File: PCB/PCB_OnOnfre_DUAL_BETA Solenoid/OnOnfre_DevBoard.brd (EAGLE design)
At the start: 44.1 x 43.8 mm, 29 parts, among them J1 9PIN 2.54MM, J3Y S8050, J7 8p, K1 G5Q-1-DC12, K2 G5Q-1-DC12, U2 esp12

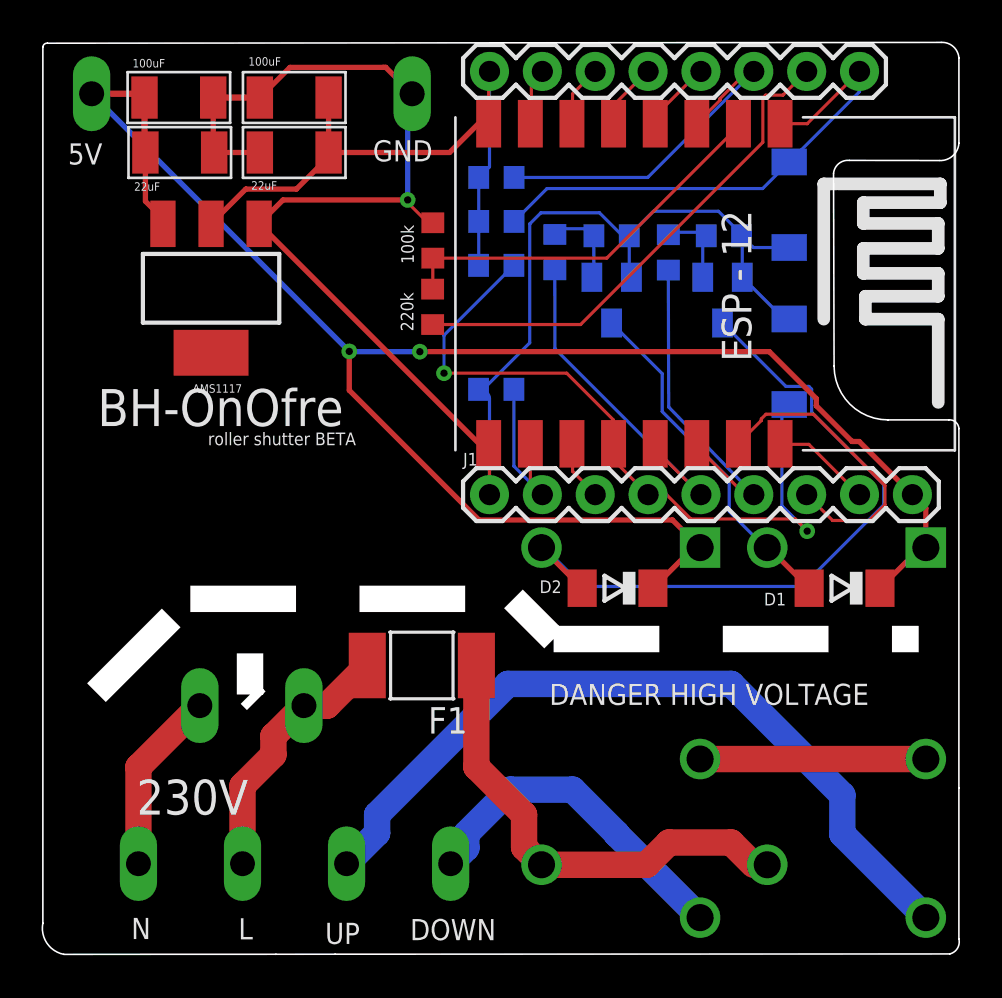
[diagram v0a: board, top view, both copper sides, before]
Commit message: s
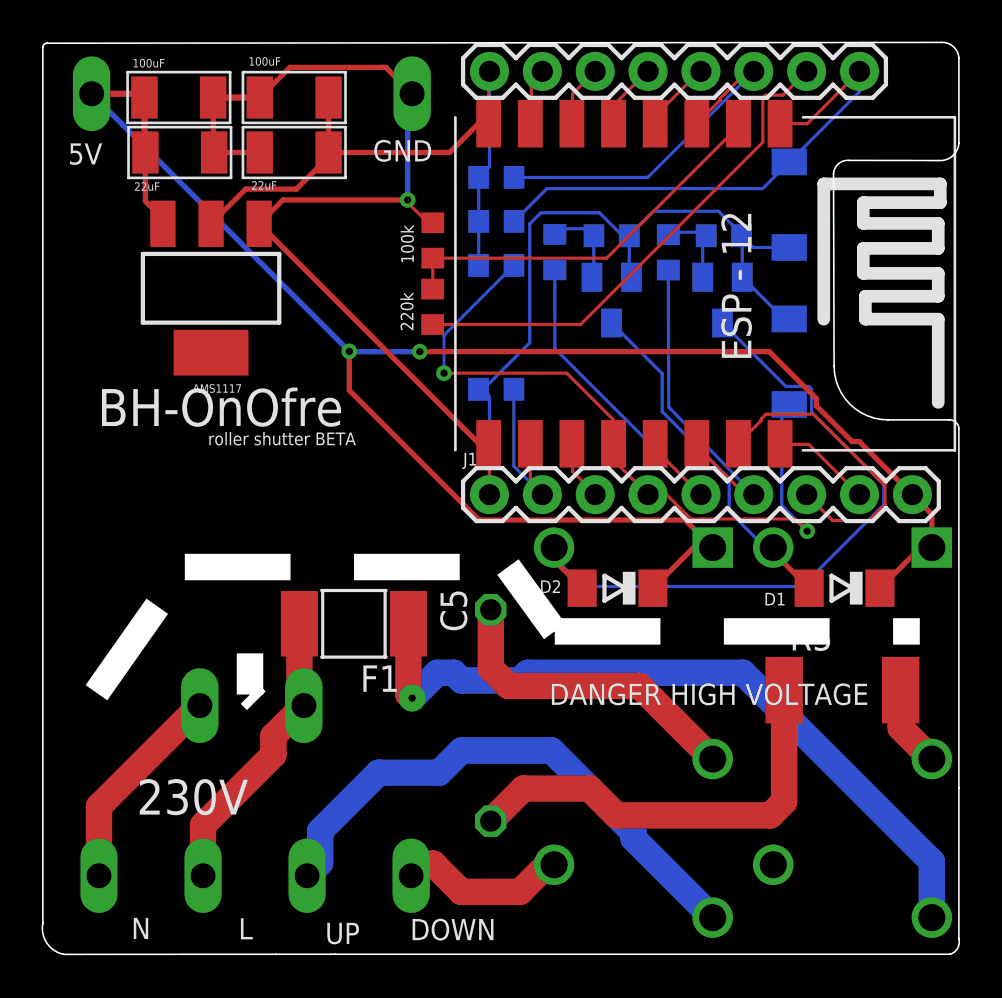
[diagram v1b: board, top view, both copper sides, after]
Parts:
- added C5: (no value), rcl:C102-043X133
- added R5: (no value), resistor:R2512
- moved F1 3.83 mm to (15.6, 18.4)
- moved X1 1.98 mm to (10.9, 5.05)
- moved K2 0.61 mm to (28.9, 13.1)
- moved K1 0.29 mm to (39.4, 13.1)
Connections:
- new net N$3: K1.2, R5.2
- new net N$4: C5.2, R5.1
- net LINE_DOWN_OUT: now also K2.4; no longer K2.3
- net LINE_IN_FUSED: now also K1.3; no longer K1.4, K2.4
- net LINE_UP_OUT: now also K2.3; no longer K1.3
- net N$2: now also C5.1; no longer K1.2
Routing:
- net N$4: track 0.00 -> 20.9 mm
- net LINE_IN_FUSED: track 21.9 -> 35.9 mm, vias 0 -> 1
- net LINE_UP_OUT: track 37.7 -> 26.4 mm
- net LINE_DOWN_OUT: track 16.4 -> 8.21 mm
- net N$2: track 10.7 -> 15.3 mm
- net N$3: track 0.00 -> 3.93 mm
- net VCC: track 88.0 -> 89.7 mm
- net LINE_L: track 12.7 -> 14.2 mm
- net NEUTRAL_IN: track 8.82 -> 10.2 mm
- net N$9: track 34.2 -> 33.6 mm
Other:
- outline, holes or cut-outs redrawn
